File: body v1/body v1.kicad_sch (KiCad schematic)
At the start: 14 parts, among them J1 Conn_02x05_Odd_Even, J2 Conn_02x05_Odd_Even, J3 Conn_02x05_Odd_Even, U1 PCF8574T, X1 XIAO-ESP32-S3-Plus-SMD

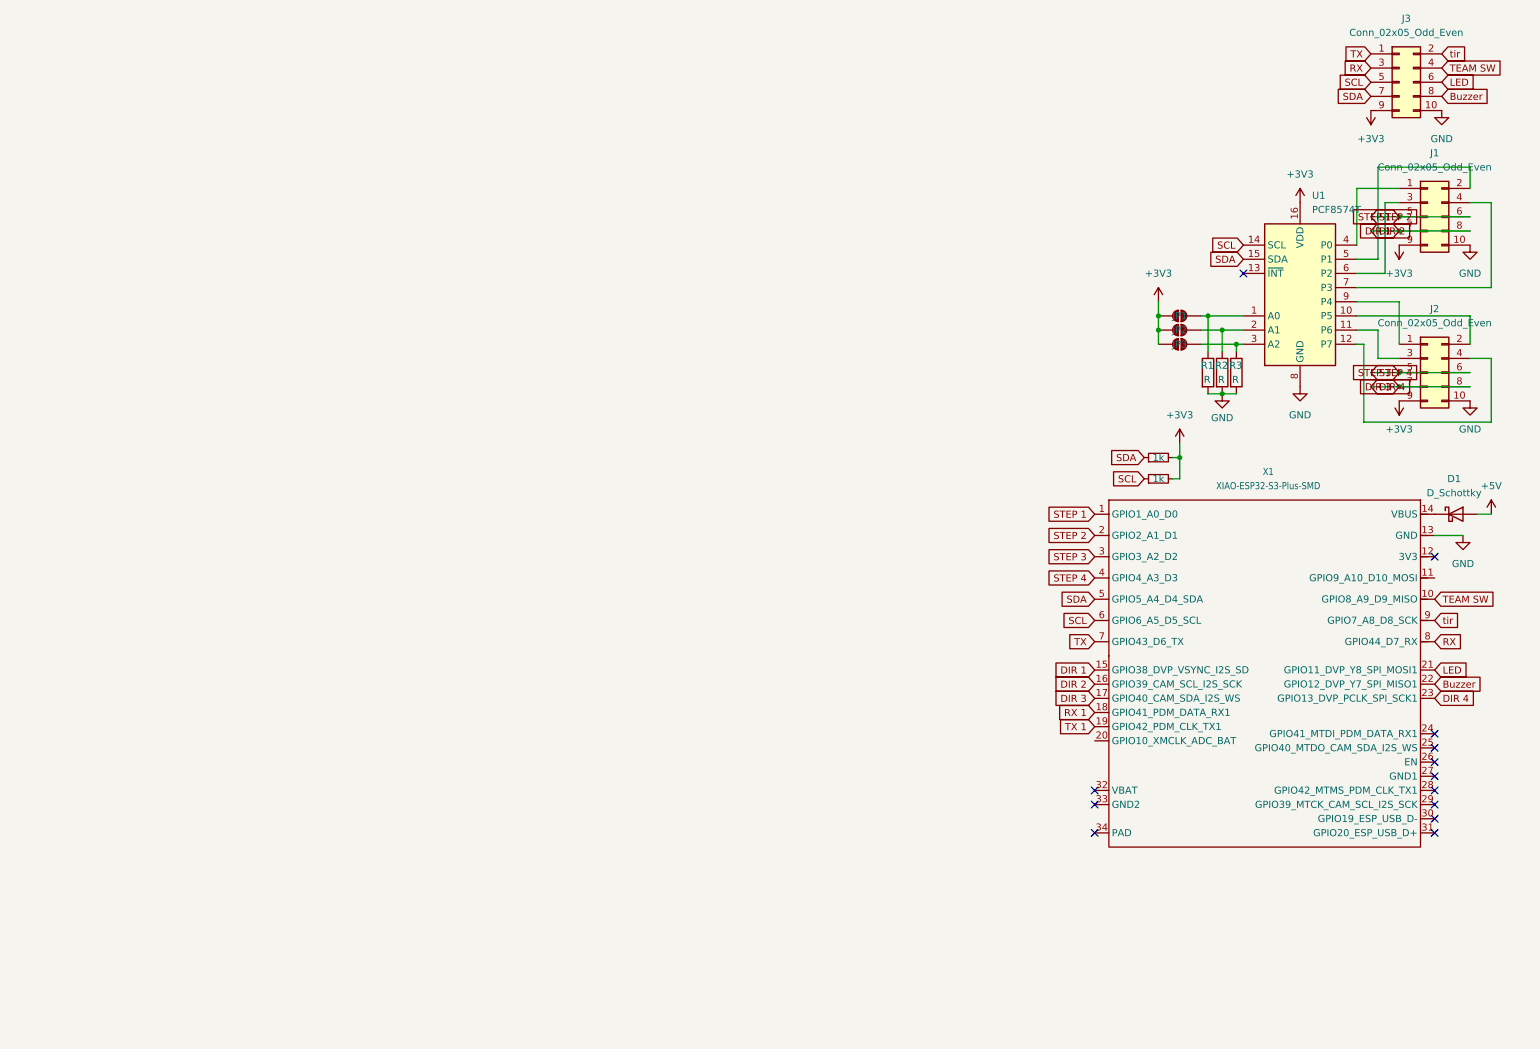
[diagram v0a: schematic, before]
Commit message: end schema body
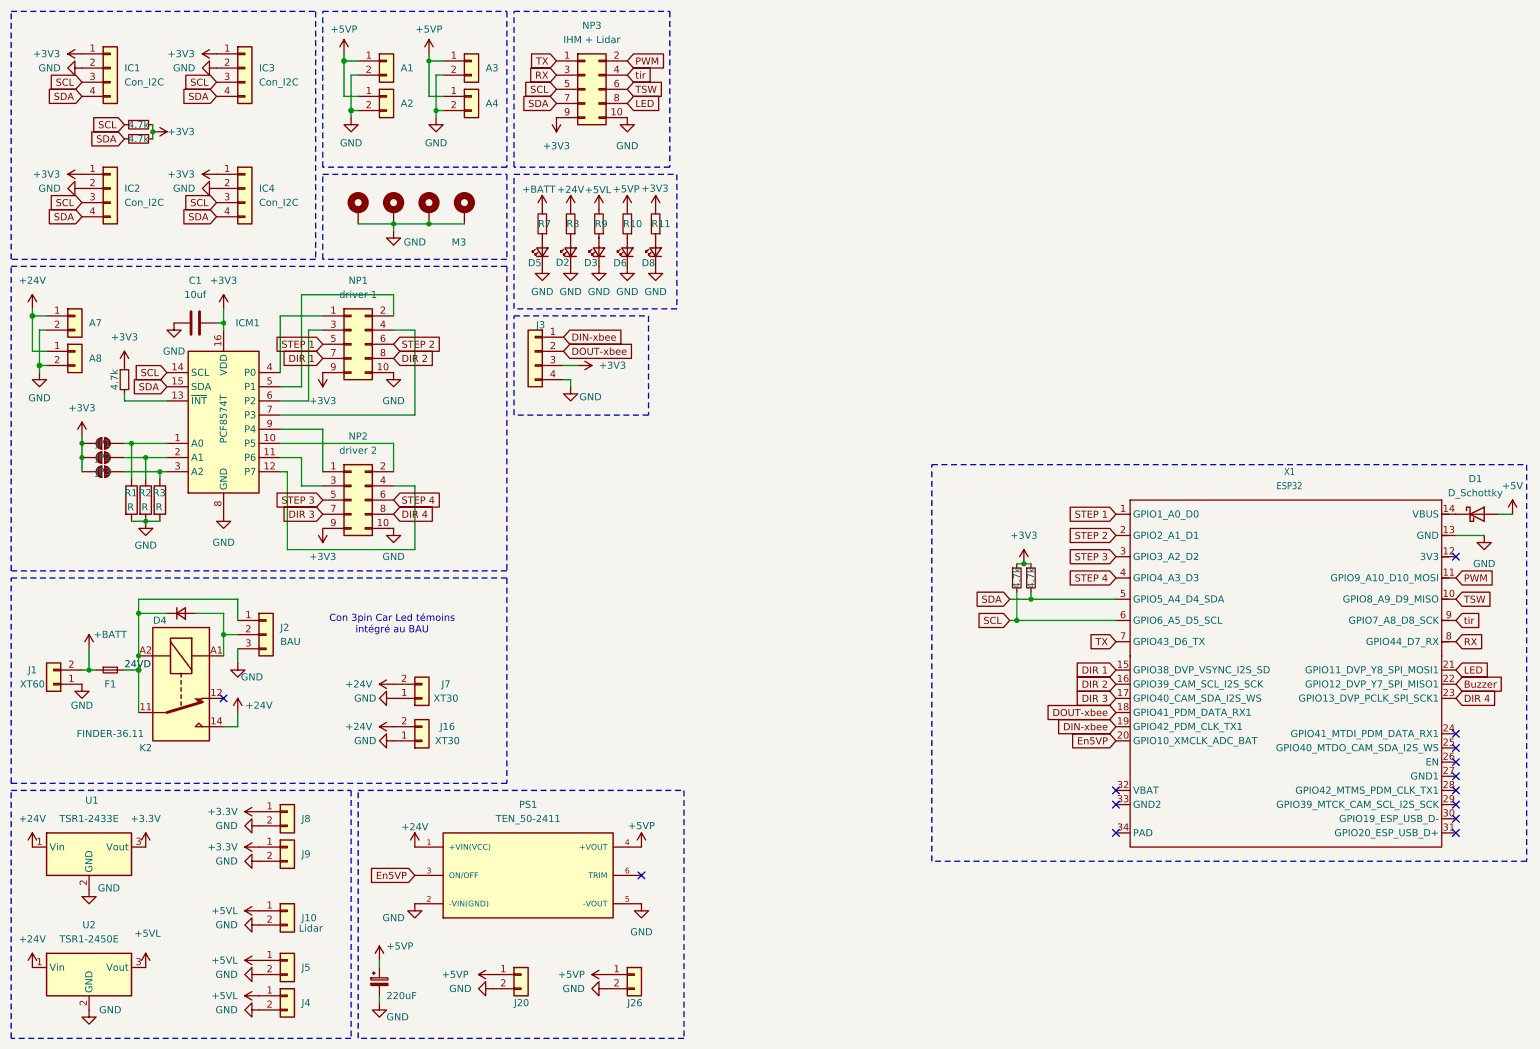
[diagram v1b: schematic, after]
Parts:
- added A1, A2, A3, A4, A7, A8: Conn_01x02, Connector_Molex:Molex_KK-254_AE-6410-02A_1x02_P2.54mm_Vertical, symbol Connector_Generic:Conn_01x02
- added C1: 10uf, Capacitor_SMD:C_1206_3216Metric_Pad1.33x1.80mm_HandSolder, symbol Device:C
- added C6: 220uF, Capacitor_THT:CP_Radial_D8.0mm_P3.80mm, symbol Device:CP_Small
- added D2, D3, D5, D6, D8: LED_Small, LED_SMD:LED_1206_3216Metric_Pad1.42x1.75mm_HandSolder, symbol Device:LED_Small
- added D4: D_Small, Diode_SMD:D_SMA_Handsoldering, symbol Device:D_Small
- added F1: Fuse_Small, Fuse:Fuseholder_Blade_Mini_Keystone_3568, symbol Device:Fuse_Small
- added H1, H2, H3, H4: M3, MountingHole:MountingHole_3.2mm_M3_Pad_Via, symbol Mechanical:MountingHole_Pad
- added IC1, IC2, IC3, IC4: Con_I2C, Connector_Molex:Molex_KK-254_AE-6410-04A_1x04_P2.54mm_Vertical, symbol Connector_Generic:Conn_01x04
- added J1: XT60, Connector_AMASS:AMASS_XT60-M_1x02_P7.20mm_Vertical, symbol Connector_Generic:Conn_01x02
- added J10: Lidar, Connector_Molex:Molex_KK-396_A-41791-0002_1x02_P3.96mm_Vertical, symbol Connector_Generic:Conn_01x02
- added J16, J7: XT30, Connector_AMASS:AMASS_XT30U-F_1x02_P5.0mm_Vertical, symbol Connector_Generic:Conn_01x02
- added J2: BAU, Connector_Molex:Molex_KK-254_AE-6410-03A_1x03_P2.54mm_Vertical, symbol Connector_Generic:Conn_01x03
- added J20, J26, J4, J5, J8, J9: ~, Connector_Molex:Molex_KK-396_A-41791-0002_1x02_P3.96mm_Vertical, symbol Connector_Generic:Conn_01x02
- added J3: Conn_01x04, Connector_Molex:Molex_KK-254_AE-6410-04A_1x04_P2.54mm_Vertical, symbol Connector_Generic:Conn_01x04
- added K2: FINDER-36.11, Relay_THT:Relay_SPDT_Finder_36.11, symbol Relay:FINDER-36.11
- added PS1: TEN_50-2411, CONV_TEN_50-2411, symbol TEN_50-2411:TEN_50-2411
- added R10, R11, R7, R8, R9: R_Small, Resistor_SMD:R_1206_3216Metric_Pad1.30x1.75mm_HandSolder, symbol Device:R_Small
- added R4, R5, R6: 4.7k, Resistor_SMD:R_1206_3216Metric_Pad1.30x1.75mm_HandSolder, symbol Device:R_Small
- added U1: TSR1-2433E, Converter_DCDC:Converter_DCDC_TRACO_TSR1-xxxxE_THT, symbol Regulator_Switching:TSR1-2433E
- added U2: TSR1-2450E, Converter_DCDC:Converter_DCDC_TRACO_TSR1-xxxxE_THT, symbol Regulator_Switching:TSR1-2450E
- JP2, JP3: footprint (none) -> Jumper:SolderJumper-2_P1.3mm_Open_RoundedPad1.0x1.5mm
- NP1: renamed from J1; value Conn_02x05_Odd_Even -> driver 1; footprint (none) -> Connector_IDC:IDC-Header_2x05_P2.54mm_Vertical
- NP2: renamed from J2; value Conn_02x05_Odd_Even -> driver 2; footprint (none) -> Connector_IDC:IDC-Header_2x05_P2.54mm_Vertical
- NP3: renamed from J3; value Conn_02x05_Odd_Even -> IHM + Lidar; footprint (none) -> Connector_IDC:IDC-Header_2x05_P2.54mm_Vertical
- R1, R2, R3: footprint (none) -> Resistor_SMD:R_1206_3216Metric_Pad1.30x1.75mm_HandSolder
- R108, R109: value 1k -> 4.7k
- X1: value XIAO-ESP32-S3-Plus-SMD -> ESP32; footprint XIAO_Series_Footprints:XIAO-ESP32-S3-Plus-SMD -> Yosh Lib:xiao s3+
- renumbered U1 to ICM1
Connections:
- net +3V3: now also R108.1, R109.1, C1.1, IC1.1 (Pin_1), IC2.1 (Pin_1), IC3.1 (Pin_1), IC4.1 (Pin_1), J3.3 (Pin_3), R11.2, R4.1, R5.1, R6.1; no longer R108.2, R109.2
- net Buzzer: no longer NP3.8 (Pin_8)
- net DIR 1: no longer NP1.8 (Pin_8), X1.16 (GPIO39_CAM_SCL_I2S_SCK)
- net DIR 3: no longer NP2.8 (Pin_8), X1.23 (GPIO13_DVP_PCLK_SPI_SCK1)
- net GND: now also A1.2 (Pin_2), A2.2 (Pin_2), A3.2 (Pin_2), A4.2 (Pin_2), A7.2 (Pin_2), A8.2 (Pin_2), C1.2, C6.2, D2.1 (K), D3.1 (K), D5.1 (K), D6.1 (K), D8.1 (K), H1.1, H2.1, H3.1, H4.1, IC1.2 (Pin_2), IC2.2 (Pin_2), IC3.2 (Pin_2), IC4.2 (Pin_2), J1.1 (Pin_1), J10.2 (Pin_2), J16.1 (Pin_1), J2.3 (Pin_3), J20.2 (Pin_2), J26.2 (Pin_2), J3.4 (Pin_4), J4.2 (Pin_2), J5.2 (Pin_2), J7.1 (Pin_1), J8.2 (Pin_2), J9.2 (Pin_2), PS1.2 (-VIN(GND)), PS1.5 (-VOUT), U1.2 (GND), U2.2 (GND)
- net LED: now also NP3.8 (Pin_8); no longer NP3.6 (Pin_6)
- net SCL: now also R109.2, IC1.3 (Pin_3), IC2.3 (Pin_3), IC3.3 (Pin_3), IC4.3 (Pin_3), R5.2; no longer R109.1
- net SDA: now also R108.2, IC1.4 (Pin_4), IC2.4 (Pin_4), IC3.4 (Pin_4), IC4.4 (Pin_4), R6.2; no longer R108.1
- net STEP 1: no longer NP1.6 (Pin_6), X1.2 (GPIO2_A1_D1)
- net STEP 3: no longer NP2.6 (Pin_6), X1.4 (GPIO4_A3_D3)
- net tir: now also NP3.4 (Pin_4); no longer NP3.2 (Pin_2)
- net at ICM1.13 (~{INT}): now also R4.2
- net PWM: now reaches X1.11 (GPIO9_A10_D10_MOSI)
- net PWM: now also NP3.2 (Pin_2)
- net En5VP: now reaches X1.20 (GPIO10_XMCLK_ADC_BAT)
- net En5VP: now also PS1.3 (ON/OFF)
- net RX 1 renamed DOUT-xbee
- net DOUT-xbee: now also J3.2 (Pin_2)
- net TEAM SW renamed TSW
- net TSW: now also NP3.6 (Pin_6); no longer NP3.4 (Pin_4)
- net TX 1 renamed DIN-xbee
- net DIN-xbee: now also J3.1 (Pin_1)
- new net: D3.2 (A), R9.1
- new net: D5.2 (A), R7.1
- new net: D8.2 (A), R11.1
- new net: D4.2 (A), J2.2 (Pin_2), K2.A1
- new net: D2.2 (A), R8.1
- new net: D6.2 (A), R10.1
- new net +24V: A7.1 (Pin_1), A8.1 (Pin_1), J16.2 (Pin_2), J7.2 (Pin_2), K2.14, PS1.1 (+VIN(VCC)), R8.2, U1.1 (Vin), U2.1 (Vin)
- new net +3.3V: J8.1 (Pin_1), J9.1 (Pin_1), U1.3 (Vout)
- new net +5VL: J10.1 (Pin_1), J4.1 (Pin_1), J5.1 (Pin_1), R9.2, U2.3 (Vout)
- new net +5VP: A1.1 (Pin_1), A2.1 (Pin_1), A3.1 (Pin_1), A4.1 (Pin_1), C6.1, J20.1 (Pin_1), J26.1 (Pin_1), PS1.4 (+VOUT), R10.2
- new net +BATT: F1.1, J1.2 (Pin_2), R7.2
- new net 24VD: D4.1 (K), F1.2, J2.1 (Pin_1), K2.11, K2.A2
- new net DIR 2: NP1.8 (Pin_8), X1.16 (GPIO39_CAM_SCL_I2S_SCK)
- new net DIR 4: NP2.8 (Pin_8), X1.23 (GPIO13_DVP_PCLK_SPI_SCK1)
- new net STEP 2: NP1.6 (Pin_6), X1.2 (GPIO2_A1_D1)
- new net STEP 4: NP2.6 (Pin_6), X1.4 (GPIO4_A3_D3)
- no-connect marks 13 -> 14
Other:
- note added: "Con 3pin Car Led témoins intégré au BAU"
- moved on the sheet: D1, ICM1, JP1, JP2, JP3, NP1, NP2, NP3, R1, R2, R3, X1

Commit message: fin schema
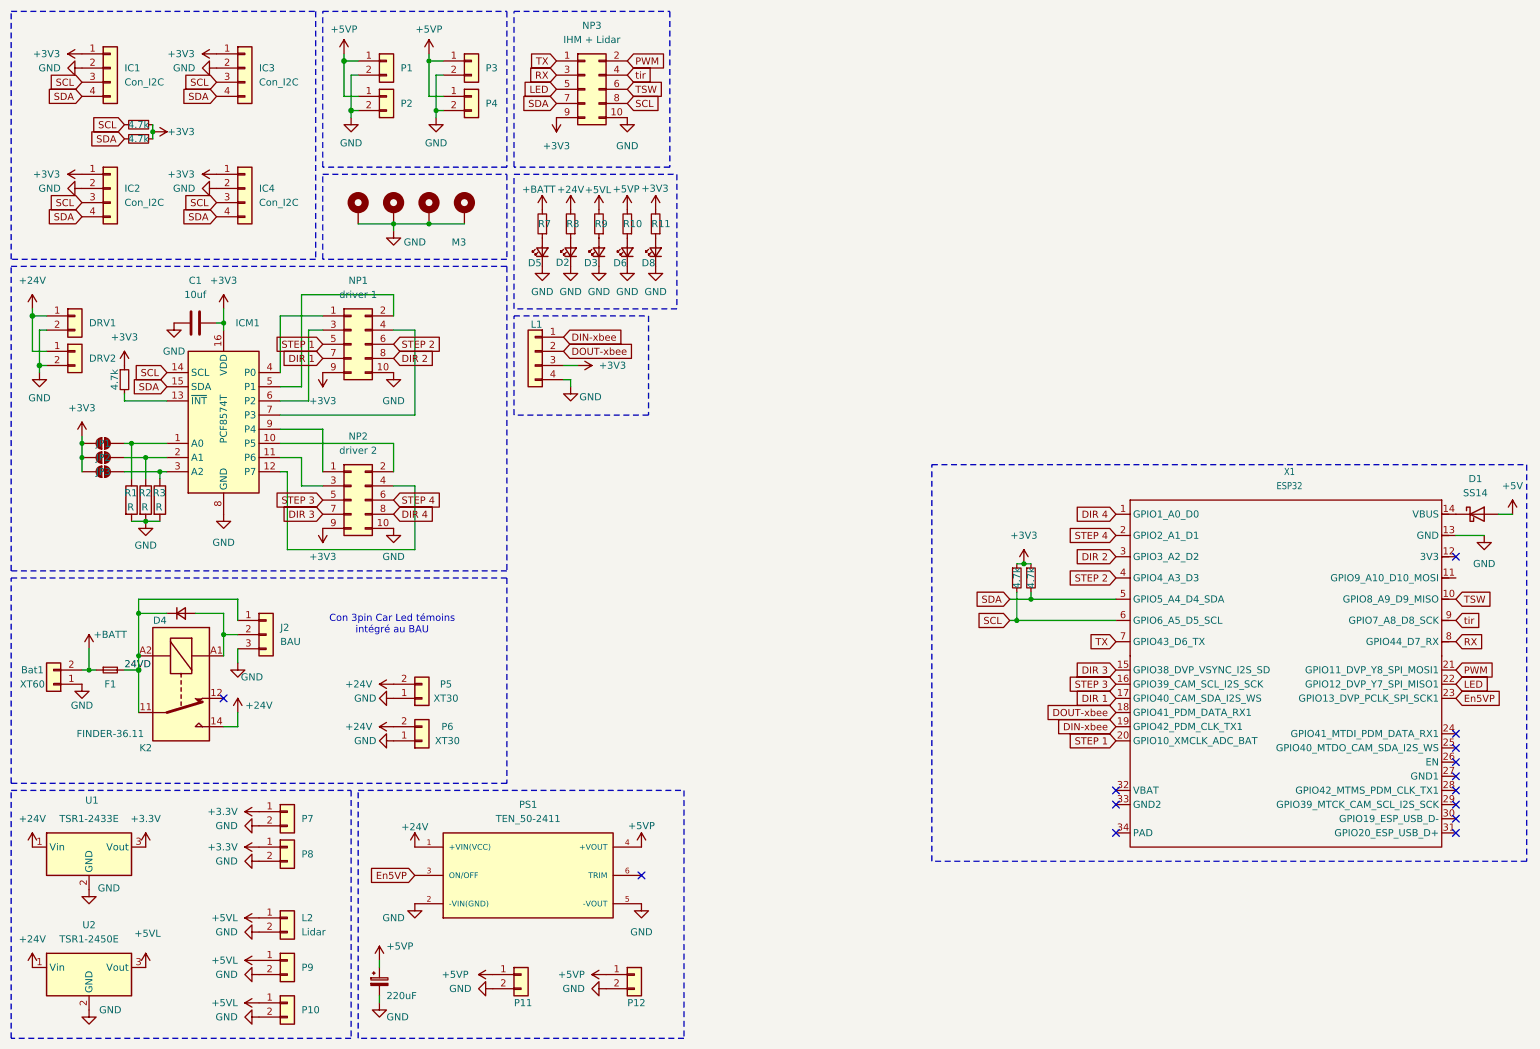
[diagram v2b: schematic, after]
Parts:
- removed D1: D_Schottky, symbol Device:D_Schottky
- added D1: SS14, Diode_SMD:D_SMA, symbol Diode:SS14
- DRV1: renamed from A7; footprint Connector_Molex:Molex_KK-254_AE-6410-02A_1x02_P2.54mm_Vertical -> Connector_AMASS:AMASS_XT30U-M_1x02_P5.0mm_Vertical
- DRV2: renamed from A8; footprint Connector_Molex:Molex_KK-254_AE-6410-02A_1x02_P2.54mm_Vertical -> Connector_AMASS:AMASS_XT30U-M_1x02_P5.0mm_Vertical
- L2: renamed from J10; footprint Connector_Molex:Molex_KK-396_A-41791-0002_1x02_P3.96mm_Vertical -> Connector_AMASS:AMASS_XT30U-M_1x02_P5.0mm_Vertical
- P1: renamed from A1; footprint Connector_Molex:Molex_KK-254_AE-6410-02A_1x02_P2.54mm_Vertical -> Connector_AMASS:AMASS_XT30U-M_1x02_P5.0mm_Vertical
- P10: renamed from J4; footprint Connector_Molex:Molex_KK-396_A-41791-0002_1x02_P3.96mm_Vertical -> Connector_AMASS:AMASS_XT30U-M_1x02_P5.0mm_Vertical
- P11: renamed from J20; footprint Connector_Molex:Molex_KK-396_A-41791-0002_1x02_P3.96mm_Vertical -> Connector_AMASS:AMASS_XT30U-M_1x02_P5.0mm_Vertical
- P12: renamed from J26; footprint Connector_Molex:Molex_KK-396_A-41791-0002_1x02_P3.96mm_Vertical -> Connector_AMASS:AMASS_XT30U-M_1x02_P5.0mm_Vertical
- P2: renamed from A2; footprint Connector_Molex:Molex_KK-254_AE-6410-02A_1x02_P2.54mm_Vertical -> Connector_AMASS:AMASS_XT30U-M_1x02_P5.0mm_Vertical
- P3: renamed from A3; footprint Connector_Molex:Molex_KK-254_AE-6410-02A_1x02_P2.54mm_Vertical -> Connector_AMASS:AMASS_XT30U-M_1x02_P5.0mm_Vertical
- P4: renamed from A4; footprint Connector_Molex:Molex_KK-254_AE-6410-02A_1x02_P2.54mm_Vertical -> Connector_AMASS:AMASS_XT30U-M_1x02_P5.0mm_Vertical
- P5: renamed from J7; footprint Connector_AMASS:AMASS_XT30U-F_1x02_P5.0mm_Vertical -> Connector_AMASS:AMASS_XT30U-M_1x02_P5.0mm_Vertical
- P6: renamed from J16; footprint Connector_AMASS:AMASS_XT30U-F_1x02_P5.0mm_Vertical -> Connector_AMASS:AMASS_XT30U-M_1x02_P5.0mm_Vertical
- P7: renamed from J8; footprint Connector_Molex:Molex_KK-396_A-41791-0002_1x02_P3.96mm_Vertical -> Connector_AMASS:AMASS_XT30U-M_1x02_P5.0mm_Vertical
- P8: renamed from J9; footprint Connector_Molex:Molex_KK-396_A-41791-0002_1x02_P3.96mm_Vertical -> Connector_AMASS:AMASS_XT30U-M_1x02_P5.0mm_Vertical
- P9: renamed from J5; footprint Connector_Molex:Molex_KK-396_A-41791-0002_1x02_P3.96mm_Vertical -> Connector_AMASS:AMASS_XT30U-M_1x02_P5.0mm_Vertical
- PS1: footprint CONV_TEN_50-2411 -> TEN 50-2411:CONV_TEN_50-2411
- renumbered J1 to Bat1, J3 to L1
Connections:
- net Buzzer is gone; now on net LED: X1.22 (GPIO12_DVP_Y7_SPI_MISO1)
- net +5V: now also D1.2 (A)
- net DIR 1: now also X1.17 (GPIO40_CAM_SDA_I2S_WS); no longer X1.15 (GPIO38_DVP_VSYNC_I2S_SD)
- net DIR 2: now also X1.3 (GPIO3_A2_D2); no longer X1.16 (GPIO39_CAM_SCL_I2S_SCK)
- net DIR 3: now also X1.15 (GPIO38_DVP_VSYNC_I2S_SD); no longer X1.17 (GPIO40_CAM_SDA_I2S_WS)
- net DIR 4: now also X1.1 (GPIO1_A0_D0); no longer X1.23 (GPIO13_DVP_PCLK_SPI_SCK1)
- net En5VP: now also X1.23 (GPIO13_DVP_PCLK_SPI_SCK1); no longer X1.20 (GPIO10_XMCLK_ADC_BAT)
- net LED: now also NP3.5 (Pin_5); no longer NP3.8 (Pin_8), X1.21 (GPIO11_DVP_Y8_SPI_MOSI1)
- net PWM: now also X1.21 (GPIO11_DVP_Y8_SPI_MOSI1); no longer X1.11 (GPIO9_A10_D10_MOSI)
- net SCL: now also NP3.8 (Pin_8); no longer NP3.5 (Pin_5)
- net STEP 1: now also X1.20 (GPIO10_XMCLK_ADC_BAT); no longer X1.1 (GPIO1_A0_D0)
- net STEP 2: now also X1.4 (GPIO4_A3_D3); no longer X1.2 (GPIO2_A1_D1)
- net STEP 3: now also X1.16 (GPIO39_CAM_SCL_I2S_SCK); no longer X1.3 (GPIO3_A2_D2)
- net STEP 4: now also X1.2 (GPIO2_A1_D1); no longer X1.4 (GPIO4_A3_D3)
- net at X1.14 (VBUS): now also D1.1 (K)
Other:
- moved on the sheet: L2, P10
